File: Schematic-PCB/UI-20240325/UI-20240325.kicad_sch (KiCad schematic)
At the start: 18 parts, among them J1 Conn_01x10_Pin, SW1 SW_Push, SW2 SW_Push, SW3 SW_Push, SW4 SW_Push, SW5 SW_Push

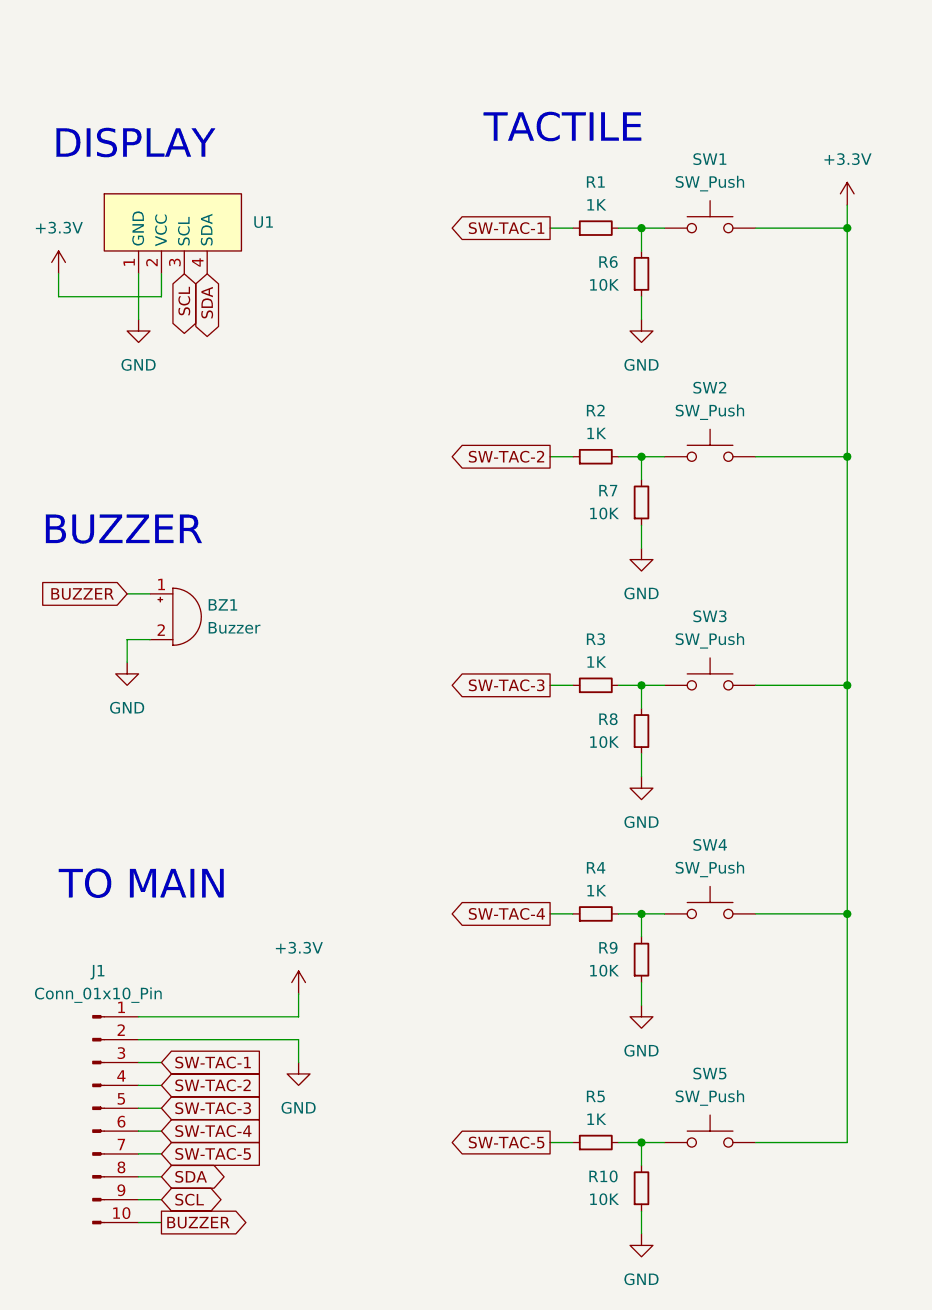
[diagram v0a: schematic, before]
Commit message: ラインセンサ基板のPCBを更新
ちょっと停滞中... ヘルプ求む、
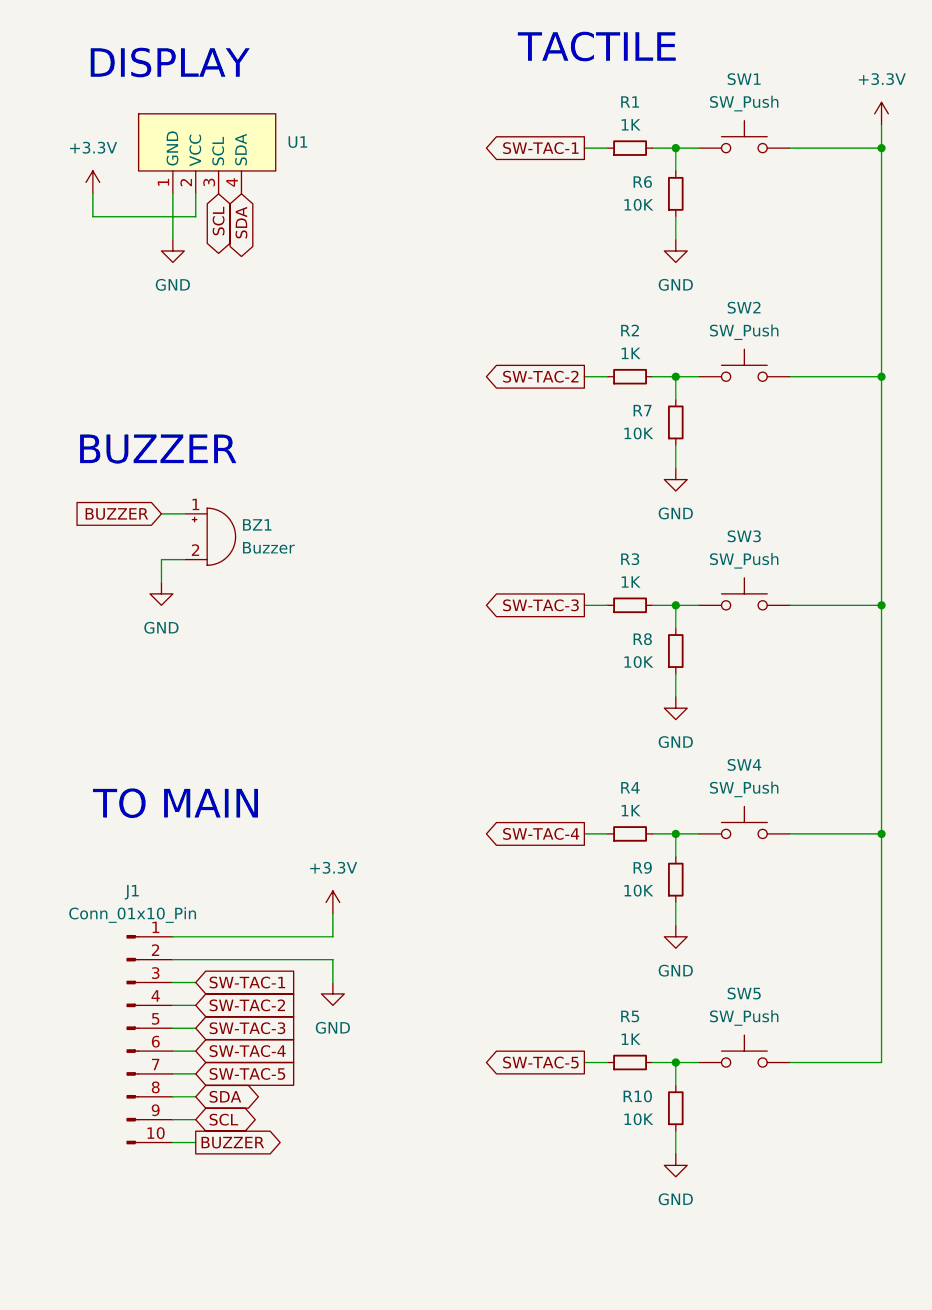
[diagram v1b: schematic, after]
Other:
- moved on the sheet: BZ1, J1, R1, R10, R2, R3, R4, R5, R6, R7, R8, R9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
